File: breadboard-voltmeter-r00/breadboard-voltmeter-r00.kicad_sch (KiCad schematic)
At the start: 2 parts, among them J1 Conn_01x04_Pin, U1 CH32V003J4M6

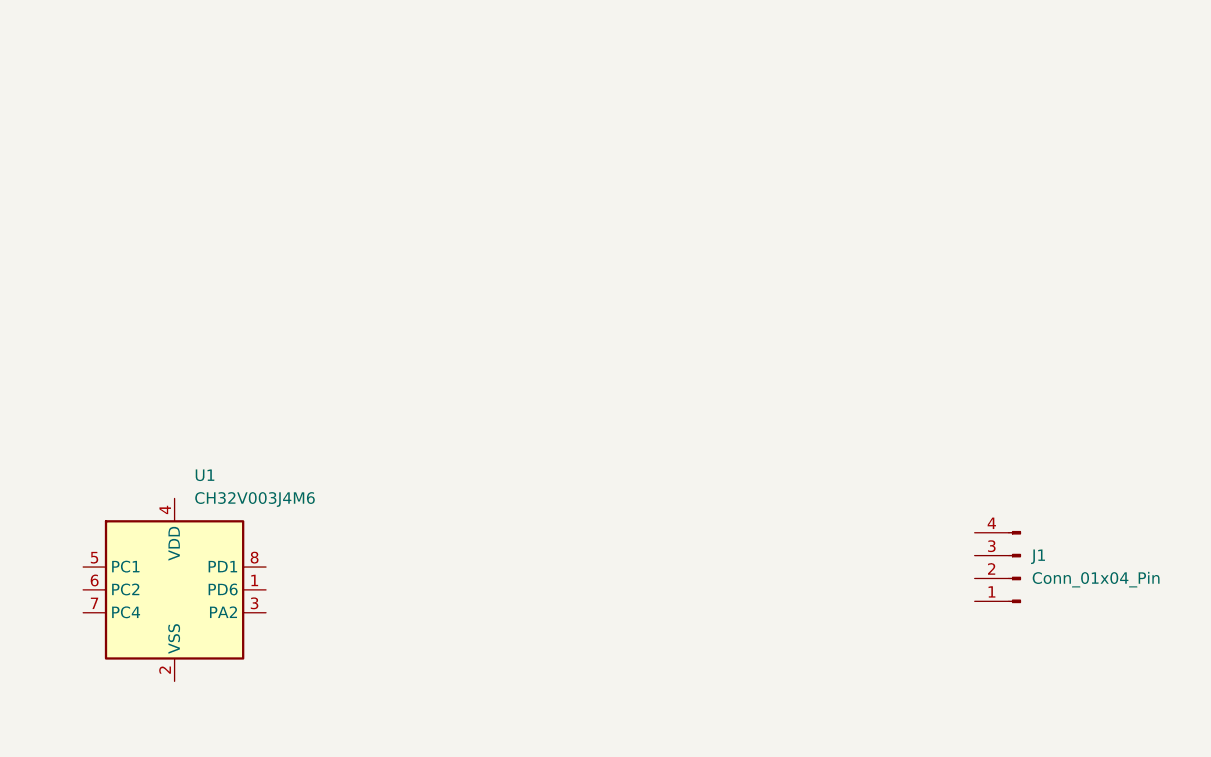
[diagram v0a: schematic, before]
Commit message: started schematics
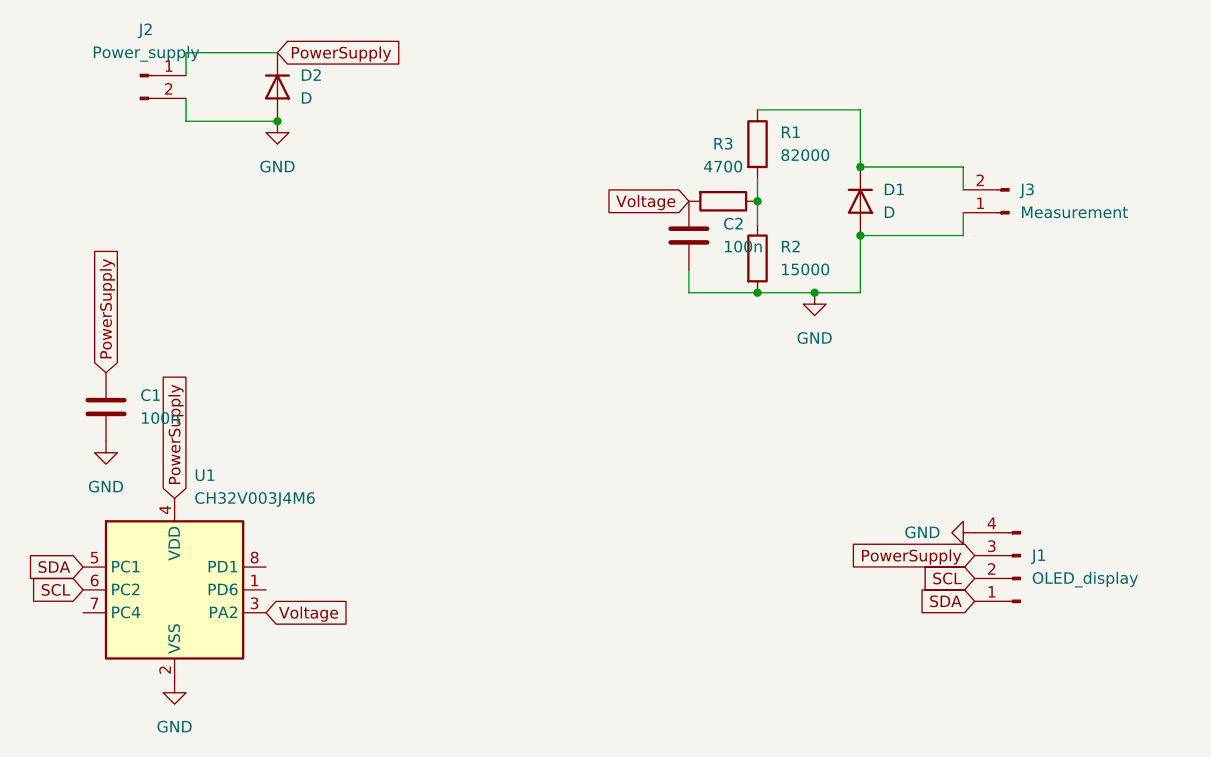
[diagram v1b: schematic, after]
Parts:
- added C1, C2: 100n, symbol Device:C
- added D1, D2: D, symbol Device:D
- added J2: Power_supply, symbol Connector:Conn_01x02_Pin
- added J3: Measurement, symbol Connector:Conn_01x02_Pin
- added R1: 82000, symbol Device:R
- added R2: 15000, symbol Device:R
- added R3: 4700, symbol Device:R
- J1: value Conn_01x04_Pin -> OLED_display
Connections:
- net GND: now reaches U1.2 (VSS)
- net GND: now also J1.4 (Pin_4), C1.2, C2.2, D1.2 (A), D2.2 (A), J2.2 (Pin_2), J3.1 (Pin_1), R2.2
- net Voltage: now reaches U1.3 (PA2)
- net Voltage: now also C2.1, R3.2
- net PowerSupply: now reaches U1.4 (VDD)
- net PowerSupply: now also J1.3 (Pin_3), C1.1, D2.1 (K), J2.1 (Pin_1)
- net SDA: now reaches U1.5 (PC1)
- net SDA: now also J1.1 (Pin_1)
- net SCL: now reaches U1.6 (PC2)
- net SCL: now also J1.2 (Pin_2)
- new net: D1.1 (K), J3.2 (Pin_2), R1.1
- new net: R1.2, R2.1, R3.1
